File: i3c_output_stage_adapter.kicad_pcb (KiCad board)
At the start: 4 copper layers, 72.5 x 50 mm, 62 parts, among them J1 PinSocket_2x12_P2.54mm_Drill1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, J2 PinSocket_2x6_P2.54mm_Drill1.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, J3 Molex_Nano-Fit_1x2_SMD_105430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, J6 JST_XH_1x3_S3B-XH-A-LF-SN, J7 PinHeader_2x10_P1.27mm_SMD, Q1 DMC31D5UDJ, Q2 DMC31D5UDJ, Q3 DMC2400UV-7, Q4 DMC2400UV-7, U1 TPS7A0518P_SOT23-5, U2 SN74LVC1G240_SC70, U3 SN74LVC1G240_SC70

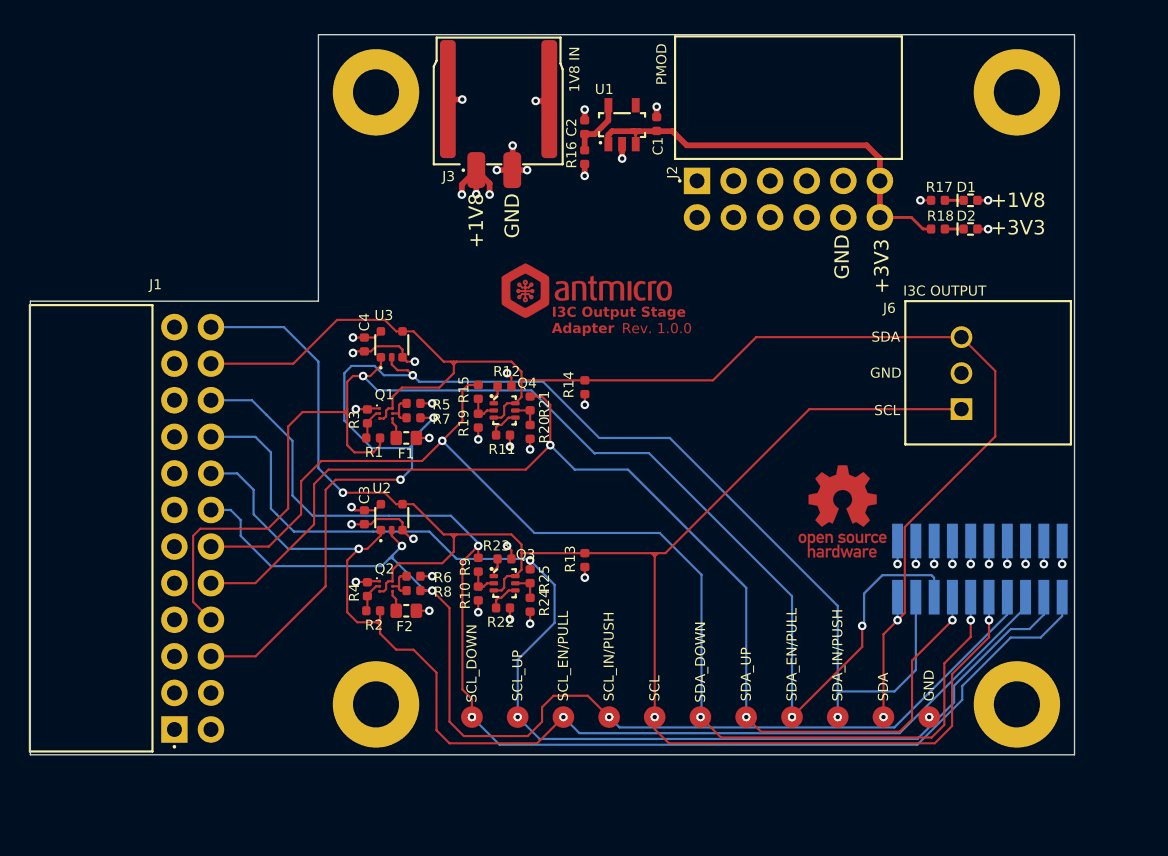
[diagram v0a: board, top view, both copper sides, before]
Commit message: [#68164] Apply changes to PCB
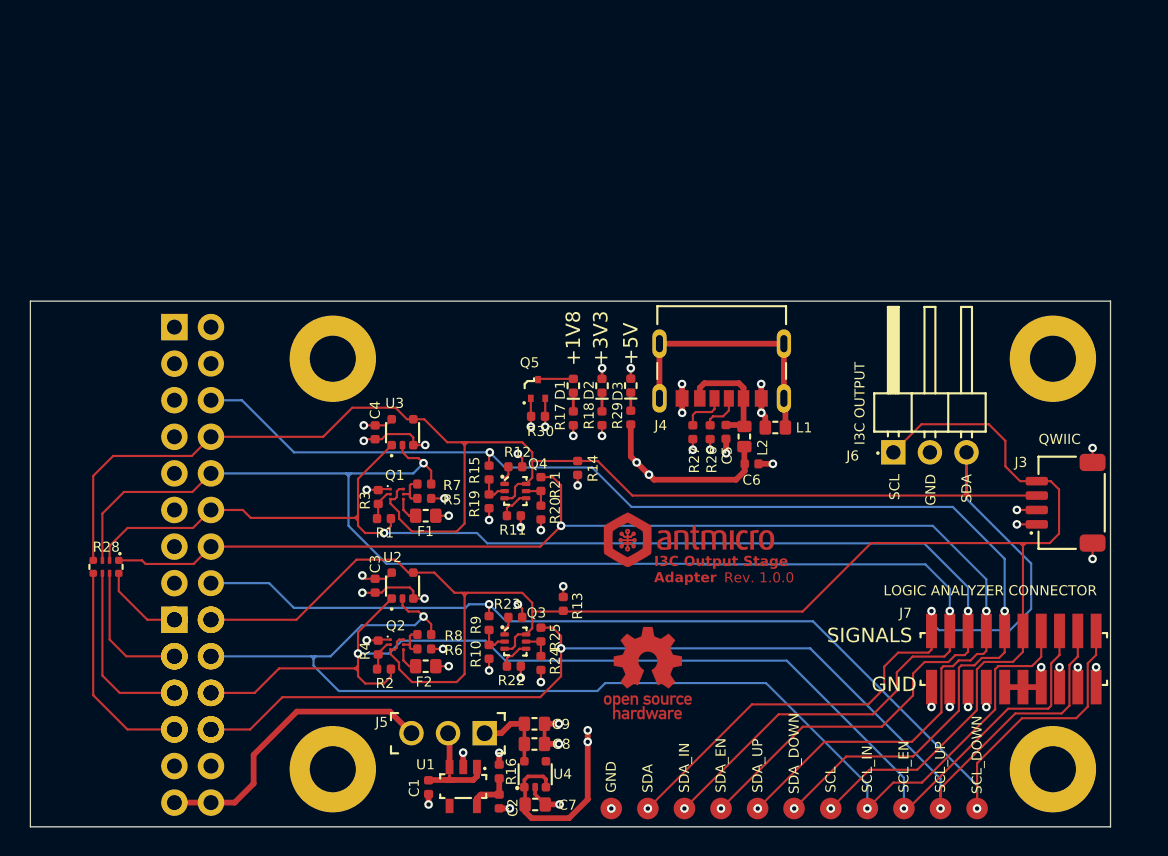
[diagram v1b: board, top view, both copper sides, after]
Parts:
- added C5: C_10n_0402, antmicro-footprints:C_0402_1005Metric, F.Cu at (148.3, 99.6)
- added C6: C_100n_16V_X7R_0402, antmicro-footprints:C_0402_1005Metric, F.Cu at (150.1, 101.8)
- added C7: C_1u_0603, antmicro-footprints:C_0603_1608Metric, F.Cu at (135.1, 125.5)
- added C8: C_1u_0603, antmicro-footprints:C_0603_1608Metric, F.Cu at (135.0, 121.2)
- added C9: C_1u_0603, antmicro-footprints:C_0603_1608Metric, F.Cu at (135.0, 119.8)
- added D3: LED_G_0402_VLMTG1500-GS08, antmicro-footprints:LED_0402_1005Metric_G, F.Cu at (141.7, 96.4)
- added J4: USB-C_CUI_UJC-HP-3-SMT-TR, antmicro-footprints:USB-C_Receptacle_CUI_UJC-HP-3-SMT-TR, F.Cu at (148.0, 94.5)
- added J5: PinHeader_1x3_P2.54mm_Drill1.1mm, antmicro-footprints:PinHeader_1x3_P2.54mm_Drill1.1mm, F.Cu at (131.5, 120.5)
- added L1: FB_120Z_2A_Murata-BLM18PG_0603, antmicro-footprints:FB_0603_1608Metric, F.Cu at (151.7, 99.3)
- added L2: FB_120Z_2A_Murata-BLM18PG_0603, antmicro-footprints:FB_0603_1608Metric, F.Cu at (149.6, 99.9)
- added Q5: DMG1012T-7, antmicro-footprints:SOT-523, F.Cu at (135.2, 96.6)
- added R26: R_5k1_0402, antmicro-footprints:R_0402_1005Metric, F.Cu at (147.2, 99.6)
- added R27: R_5k1_0402, antmicro-footprints:R_0402_1005Metric, F.Cu at (146.0, 99.6)
- added R28: 4x0R_0402_array, antmicro-footprints:4x0R_0402_array_EXB28V, F.Cu at (105.2, 109.0)
- added R29: R_2k_0402, antmicro-footprints:R_0402_1005Metric, F.Cu at (141.7, 98.6)
- added R30: R_10k_0402, antmicro-footprints:R_0402_1005Metric, F.Cu at (135.2, 98.5)
- added REF**: Jumper_1x2_P2.54mm, antmicro-footprints:Jumper_1x2_P2.54mm, F.Cu at (129.0, 120.5)
- added U4: TLV70033_SC70, antmicro-footprints:SC-70-5, F.Cu at (135.1, 123.4)
- J1, J2: moved to B.Cu
- J3: value Molex_Nano-Fit_1x2_SMD_1054301202 -> JST_SH_1x4_SM04B-SRSS-TB-LF-SN; footprint antmicro-footprints:Conn_Molex_Nano-Fit_1x2_SMD_1054301202 -> antmicro-footprints:Conn_JST_SH_1x4_SM04B-SRSS-TB-LF-SN
- J6: value JST_XH_1x3_S3B-XH-A-LF-SN -> PinHeader_1x3_P2.54mm_Drill1.1mm_Horizontal; footprint antmicro-footprints:Conn_JST_XH_1x3_S3B-XH-A-LF-SN -> antmicro-footprints:PinHeader_1x3_P2.54mm_Horizontal
- J7: moved to F.Cu
- moved C1 48.7 mm to (127.7, 124.2), turned to 90 degrees
- moved J3 48.4 mm to (172.0, 104.5), turned to 90 degrees
- moved J2 47.4 mm to (110.0, 112.6), turned to -90 degrees
- moved U1 47.3 mm to (130.1, 124.2), turned to -90 degrees
- moved C2 47.2 mm to (132.6, 125.2), turned to 90 degrees
- moved R16 43.1 mm to (132.6, 123.2), turned to 90 degrees
- moved TP11 35.6 mm to (165.7, 125.7)
- moved D1 30.4 mm to (137.7, 96.4), turned to -90 degrees
- moved TP10 30.0 mm to (163.2, 125.7)
- moved R17 29.5 mm to (137.7, 98.6), turned to -90 degrees
- moved J1 27.9 mm to (110.0, 92.3), turned to -90 degrees
- moved D2 27.8 mm to (139.7, 96.4), turned to -90 degrees
- moved R18 26.8 mm to (139.7, 98.6), turned to -90 degrees
- moved TP9 24.5 mm to (160.7, 125.7)
- moved TP1 23.0 mm to (140.3, 125.7)
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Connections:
- D1 pad 1: GND -> Net-(D1-C)
- J1 pad 10: /SDA_UP -> /SDA_IN/PUSH
- J1 pad 12: /SDA_DOWN -> /SDA_EN/PULL
- J1 pad 14: /SCL_IN/PUSH -> /SDA_UP
- J1 pad 16: /SCL_EN/PULL -> /SCL_DOWN
- J1 pad 17: GND -> /PMOD1
- J1 pad 18: /SCL_UP -> /SCL
- J1 pad 19: GND -> /PMOD3
- J1 pad 20: /SCL_DOWN -> /SCL_IN/PUSH
- J1 pad 21: GND -> /PMOD5
- J1 pad 22: /SDA -> /SCL_EN/PULL
- J1 pad 23: GND -> /PMOD7
- J1 pad 24: /SCL -> /SCL_UP
- J1 pad 6: /SDA_IN/PUSH -> /SDA_DOWN
- J1 pad 8: /SDA_EN/PULL -> /SDA
- J2 pad 1: unconnected-(J2-Pad1) -> /PMOD1
- J2 pad 11: +3V3 -> /PMOD_3V3
- J2 pad 12: +3V3 -> /PMOD_3V3
- J2 pad 2: unconnected-(J2-Pad2) -> /SCL
- J2 pad 3: unconnected-(J2-Pad3) -> /PMOD3
- J2 pad 4: unconnected-(J2-Pad4) -> /SCL_IN/PUSH
- J2 pad 5: unconnected-(J2-Pad5) -> /PMOD5
- J2 pad 6: unconnected-(J2-Pad6) -> /SCL_EN/PULL
- J2 pad 7: unconnected-(J2-Pad7) -> /PMOD7
- J2 pad 8: unconnected-(J2-Pad8) -> /SCL_UP
- J3 pad 1: +1V8 -> GND
- J3 pad 2: GND -> +3V3
- R17 pad 2: +1V8 -> +3V3
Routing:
- net +5V: track 0.00 -> 49.5 mm, vias 0 -> 4
- net /SDA: track 101.4 -> 147.5 mm
- net +3V3: track 30.1 -> 69.7 mm, vias 0 -> 3
- net /PMOD_3V3: track 0.00 -> 20.9 mm
- net GNDREF: track 0.00 -> 18.3 mm
- net /PMOD7: track 0.00 -> 15.1 mm
- net /PMOD5: track 0.00 -> 12.6 mm
- net /SDA_UP: track 82.2 -> 94.6 mm
- net GND: track 43.4 -> 54.8 mm, vias 31 -> 39
- net /PMOD3: track 0.00 -> 9.58 mm
- net Net-(C5-Pad1): track 0.00 -> 8.06 mm
- net /SDA_IN/PUSH: track 100.2 -> 106.7 mm, vias 4 -> 3
- net /SCL_DOWN: track 85.9 -> 79.6 mm
- net /SCL_IN/PUSH: track 78.5 -> 84.6 mm, vias 3 -> 2
- net /PMOD1: track 0.00 -> 5.92 mm
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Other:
- board size 72.5 x 50 mm -> 75 x 36.5 mm
- board text added: "+5V"
- board text added: "QWIIC"
- board text added: "SCL_EN"
- board text added: "SCL_IN"
- board text added: "SDA_EN"
- board text added: "SDA_IN"
- board text removed: "1V8 IN"
- board text removed: "PMOD"
- board text removed: "SCL_EN/PULL"
- board text removed: "SCL_IN/PUSH"
- board text removed: "SDA_EN/PULL"
- board text removed: "SDA_IN/PUSH"
